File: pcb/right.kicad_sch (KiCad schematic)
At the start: 47 parts, among them J1 OLED Connector, J2 Tag connect TC2030-CTX, J4 Conn_01x01_Socket, J5 Conn_01x01_Socket, SW1 RESET, SW23 EC11 Encoder, SW24 ON/OFF, U1 nRF52840, U4 DRV2605LDGS, Y1 32MHz, Y2 32.768kHz

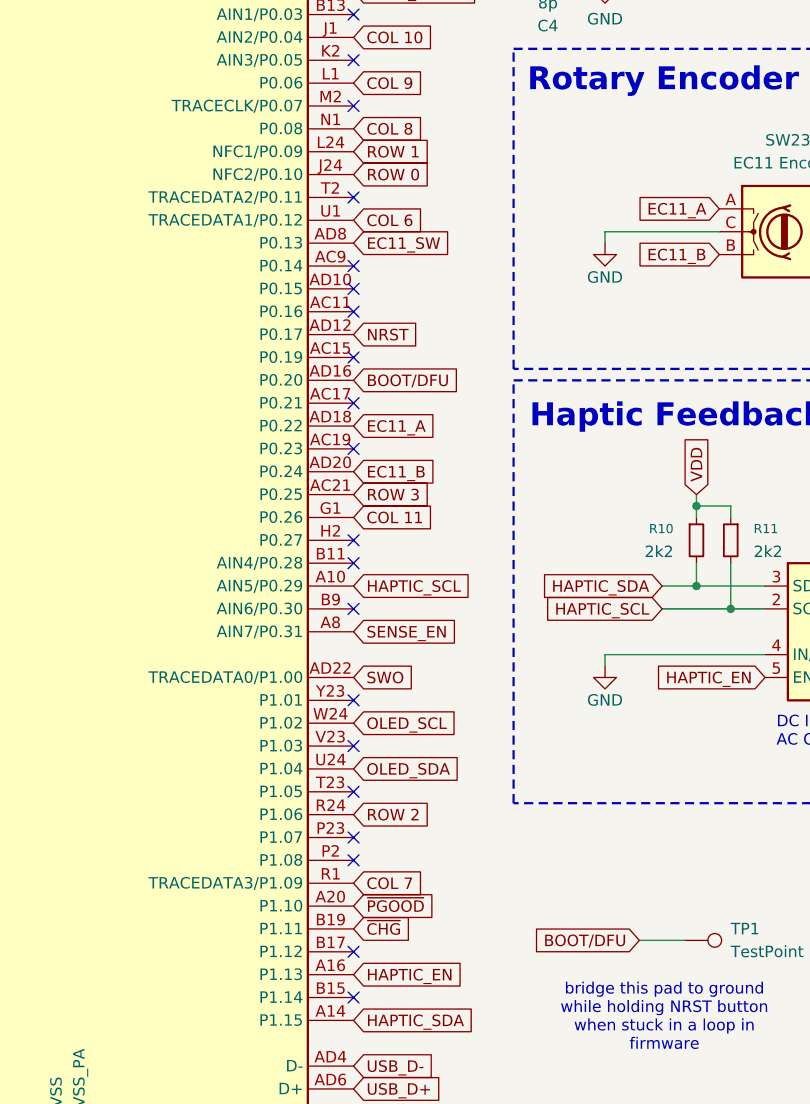
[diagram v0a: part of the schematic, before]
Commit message: finished routing second half
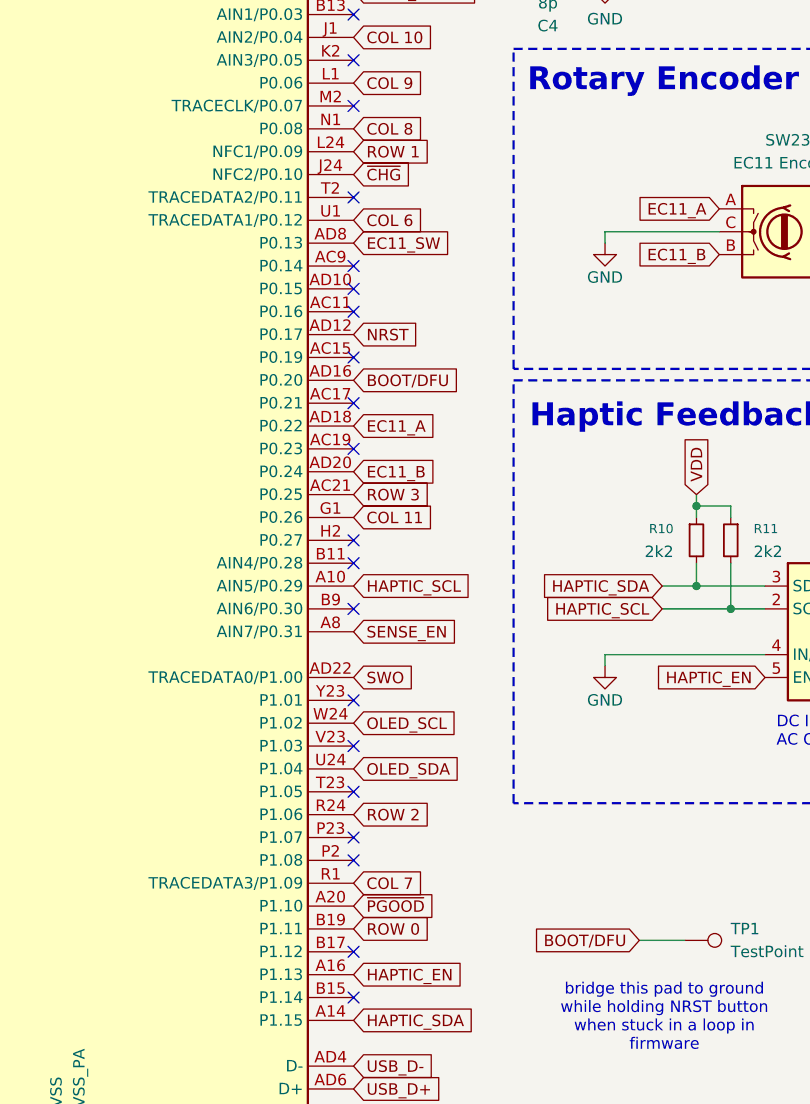
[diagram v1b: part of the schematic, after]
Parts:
- H1, H2, H3, H4, H5: footprint (none) -> MountingHole:MountingHole_2.2mm_M2
- J1, SW23: price (none) -> 0.90
- J4, J5: price (none) -> 0.03
- SW1: price (none) -> 0.05
- SW24: price (none) -> 0.07
- U1: price (none) -> 6.00
- U4: price (none) -> 1.18
- Y1: price (none) -> 0.12
- Y2: price (none) -> 0.17
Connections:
- net ROW 0: now also U1.B19 (P1.11); no longer U1.J24 (NFC2/P0.10)
- net ~{CHG}: now also U1.J24 (NFC2/P0.10); no longer U1.B19 (P1.11)
